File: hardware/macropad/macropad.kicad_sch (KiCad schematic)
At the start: 33 parts, among them J1 SWD, J2 USB_C_Receptacle_USB2.0_16P, J3 Conn_01x02, J4 display(4x1), J6 Enc2, J7 Enc1, SW1 SW_Push, SW2 SW_Push, SW3 SW_Push, SW4 SW_Push, SW5 SW_Push, SW6 SW_Push, SW7 SW_Push, SW8 SW_Push, SW9 SW_Push, U2 STM32F103C8Tx, U3 NRF24L01_Breakout, Y1 8Mhz C_L=12pF

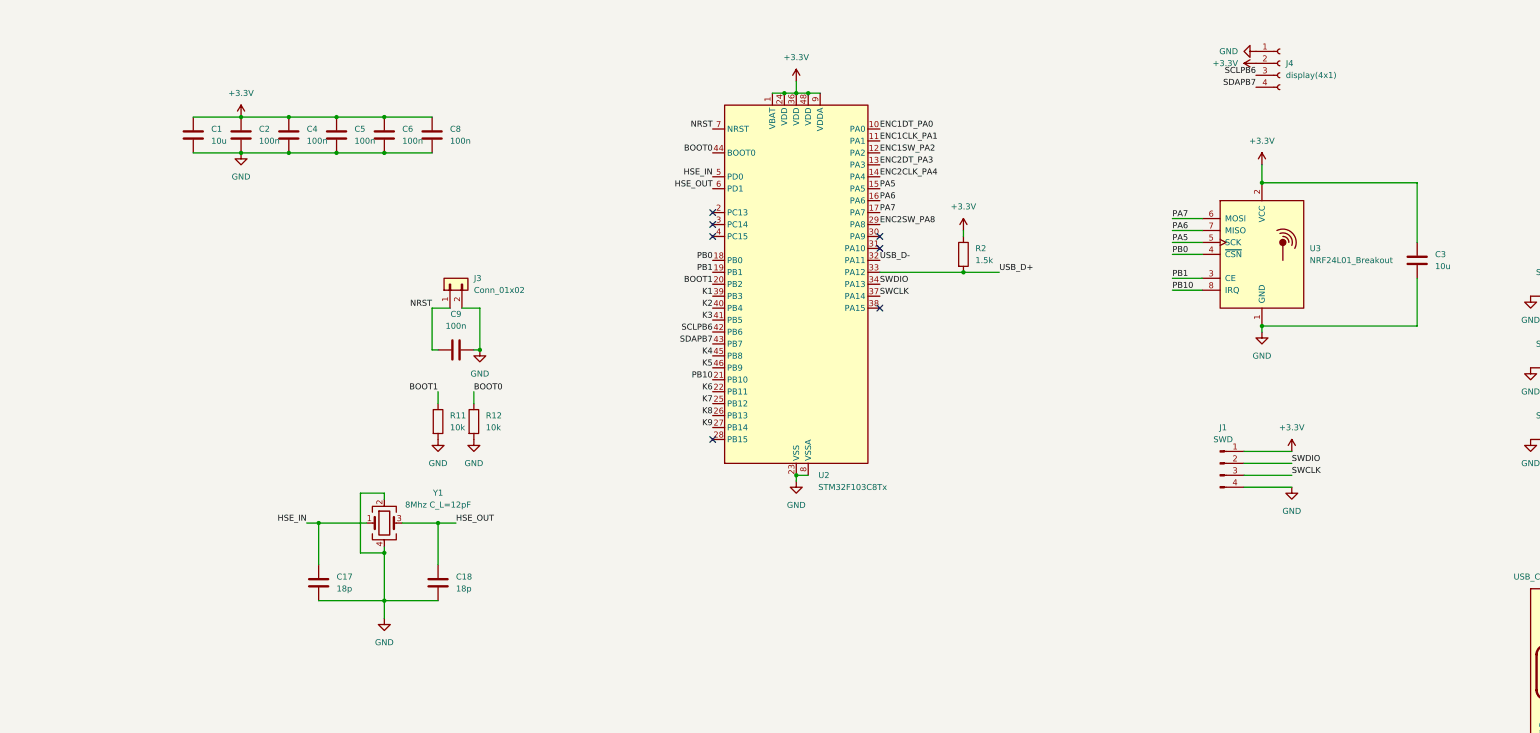
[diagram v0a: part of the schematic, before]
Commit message: updated. comments in whatsapp
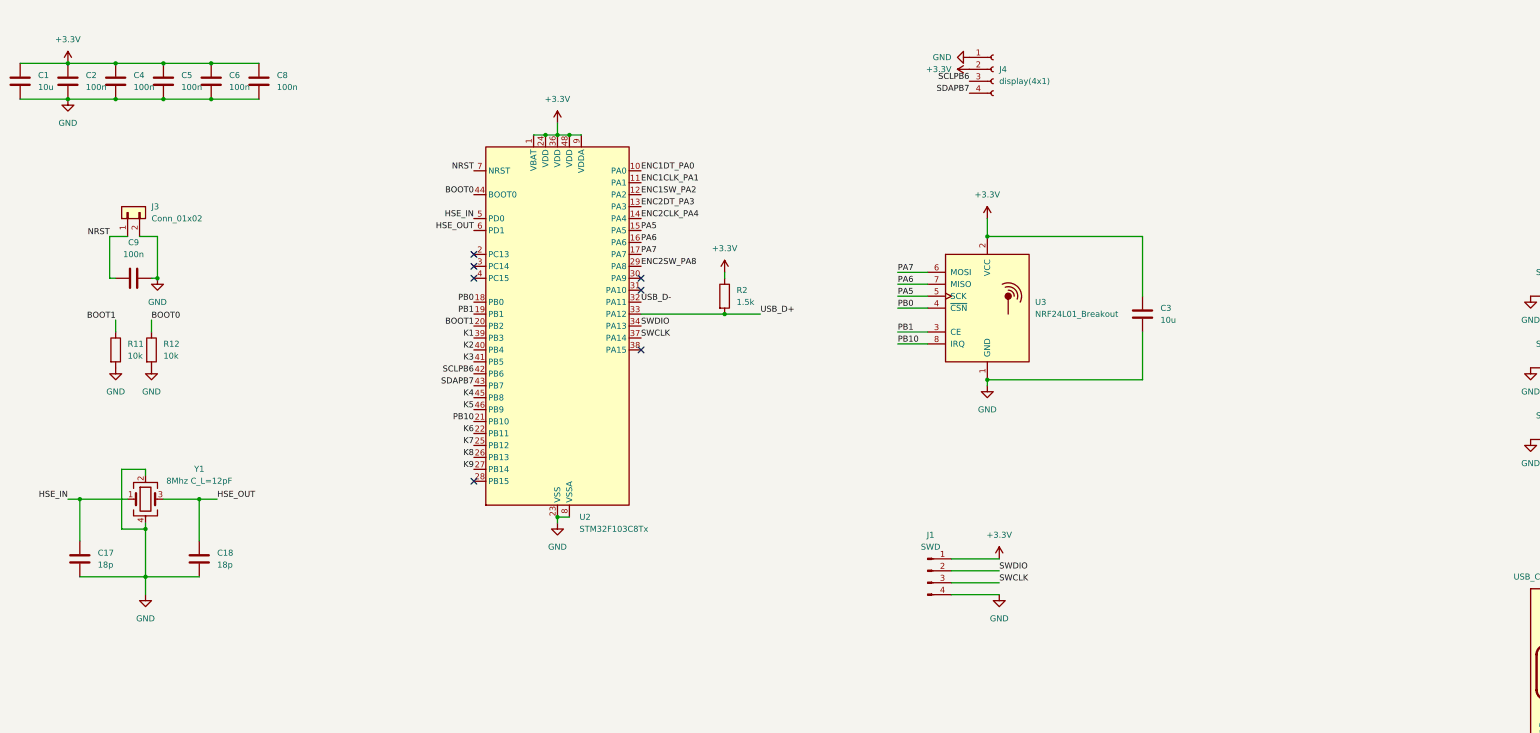
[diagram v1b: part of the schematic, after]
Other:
- moved on the sheet: C1, C17, C18, C2, C3, C4, C5, C6, C8, C9, J1, J3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
